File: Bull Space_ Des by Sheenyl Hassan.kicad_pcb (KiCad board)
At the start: 2 copper layers, 20 parts, among them IC1 TEENSY_4.0, IC2 XB24CZ7PIT-004, J1 Screw_Terminal_01x02, J2 Screw_Terminal_01x02, U1 Regulator_Linear_AP2204RB-3.3, U2 Flight-Computer_Adafruit_GPS_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, U3 ADXL343, U4 BMP280, U6 Memory_Flash_W25Q32JVSS

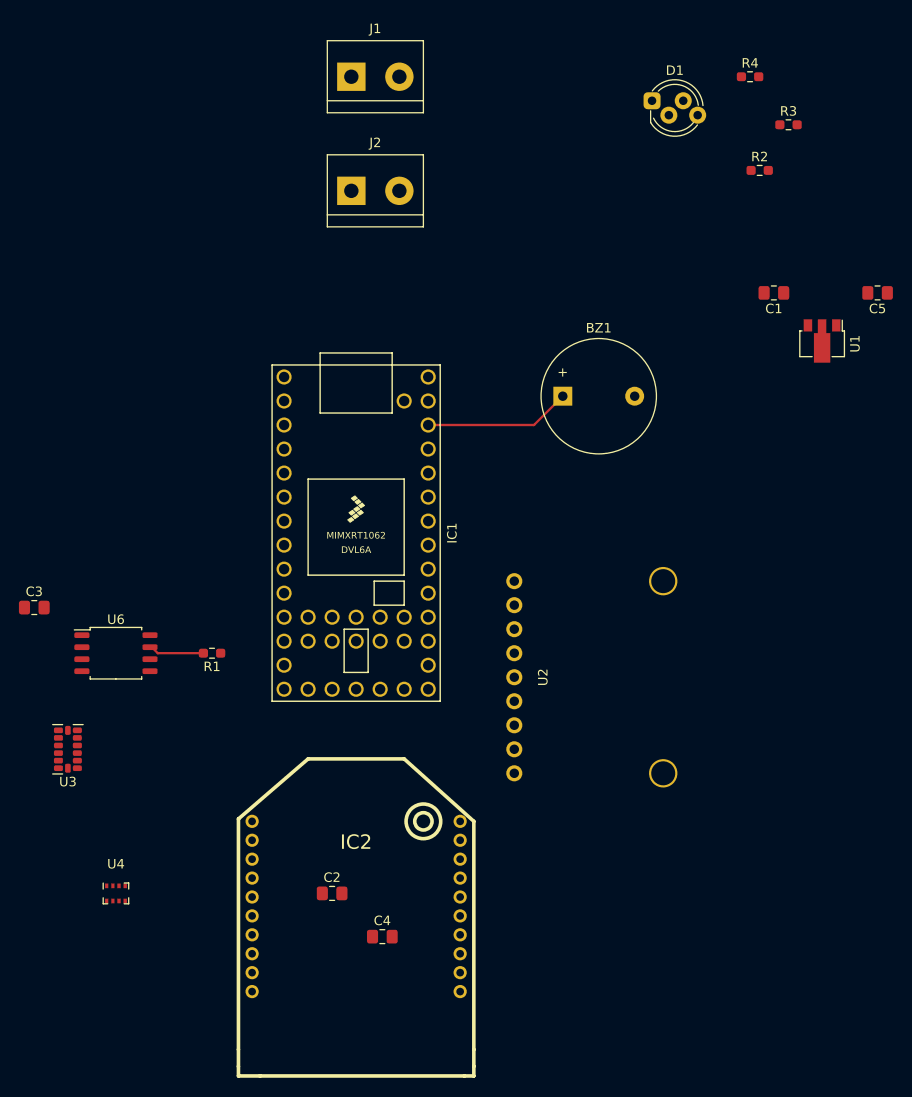
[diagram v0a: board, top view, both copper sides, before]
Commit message: Board Layout (kinda)
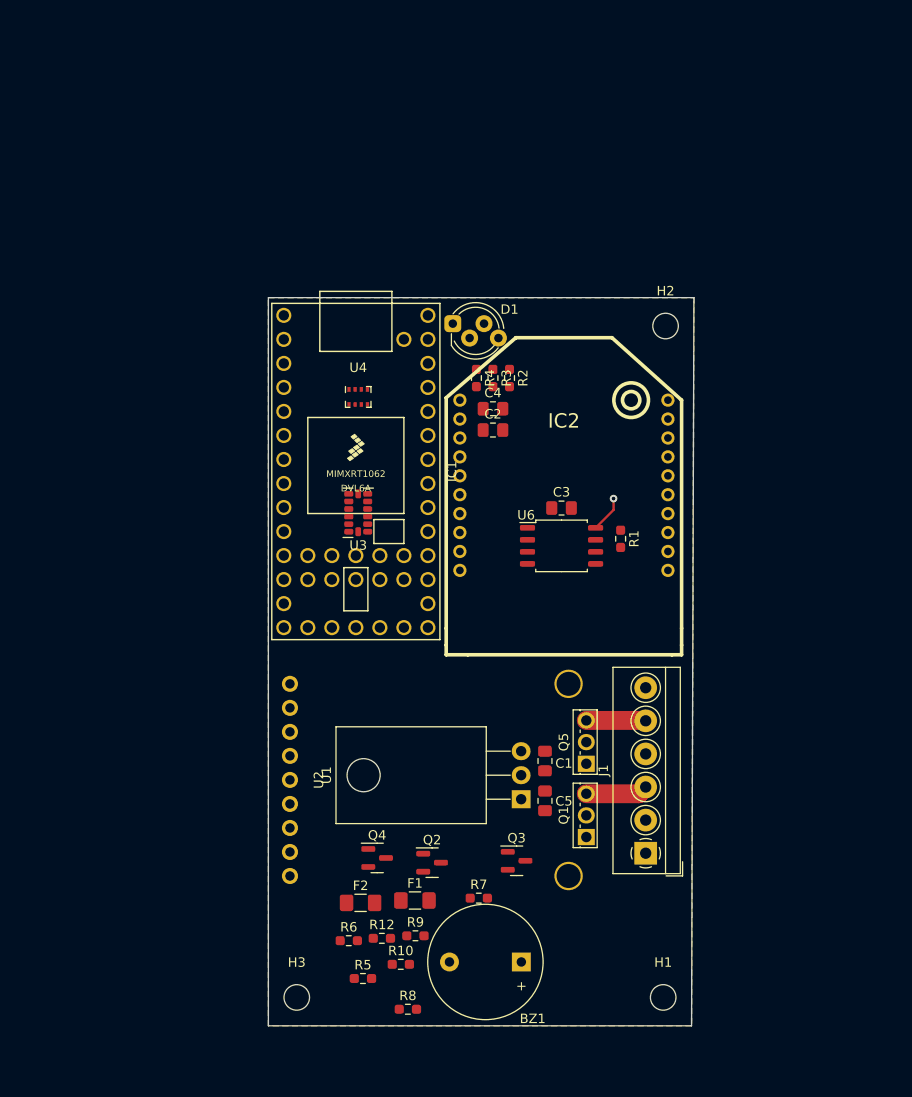
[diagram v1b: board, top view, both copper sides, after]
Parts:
- removed J2: Screw_Terminal_01x02, TerminalBlock:TerminalBlock_bornier-2_P5.08mm
- added F1: 3A Polyfuse, Fuse:Fuse_1206_3216Metric_Pad1.42x1.75mm_HandSolder, F.Cu at (87.5, 127.8)
- added F2: 3A Polyfuse, Fuse:Fuse_1206_3216Metric_Pad1.42x1.75mm_HandSolder, F.Cu at (81.8, 128.0)
- added H1: MountingHole, MountingHole:MountingHole_2.7mm_M2.5, F.Cu at (113.8, 138.0)
- added H2: MountingHole, MountingHole:MountingHole_2.7mm_M2.5, F.Cu at (114.0, 67.0)
- added H3: MountingHole, MountingHole:MountingHole_2.7mm_M2.5, F.Cu at (75.0, 138.0)
- added Q1: AOI21357, Package_TO_SOT_THT:TO-251-3_Vertical, F.Cu at (105.6, 121.0)
- added Q2: 2N7002, Package_TO_SOT_SMD:SOT-23, F.Cu at (89.3, 123.8)
- added Q3: 2N7002, Package_TO_SOT_SMD:SOT-23, F.Cu at (98.2, 123.5)
- added Q4: 2N7002, Package_TO_SOT_SMD:SOT-23, F.Cu at (83.5, 123.2)
- added Q5: AOI21357, Package_TO_SOT_THT:TO-251-3_Vertical, F.Cu at (105.6, 113.3)
- added R10: 10k, Resistor_SMD:R_0603_1608Metric_Pad0.98x0.95mm_HandSolder, F.Cu at (86.0, 134.5)
- added R12: 10k, Resistor_SMD:R_0603_1608Metric_Pad0.98x0.95mm_HandSolder, F.Cu at (84.0, 131.8)
- added R5: 100R, Resistor_SMD:R_0603_1608Metric_Pad0.98x0.95mm_HandSolder, F.Cu at (82.0, 136.0)
- added R6: 100R, Resistor_SMD:R_0603_1608Metric_Pad0.98x0.95mm_HandSolder, F.Cu at (80.5, 132.0)
- added R7: 100, Resistor_SMD:R_0603_1608Metric_Pad0.98x0.95mm_HandSolder, F.Cu at (94.2, 127.5)
- added R8: 10k, Resistor_SMD:R_0603_1608Metric_Pad0.98x0.95mm_HandSolder, F.Cu at (86.8, 139.2)
- added R9: 10k, Resistor_SMD:R_0603_1608Metric_Pad0.98x0.95mm_HandSolder, F.Cu at (87.5, 131.5)
- C1: value 1uf -> 10uf
- J1: value Screw_Terminal_01x02 -> Screw_Terminal_01x06; footprint TerminalBlock:TerminalBlock_bornier-2_P5.08mm -> TerminalBlock_4Ucon:TerminalBlock_4Ucon_1x06_P3.50mm_Horizontal
- U1: value Regulator_Linear_AP2204RB-3.3 -> VXO7803-1000; footprint Package_TO_SOT_SMD:SOT-89-3 -> Package_TO_SOT_THT:TO-220-3_Horizontal_TabDown
- U2: footprint Flight Computer:Adafruit_ADXL345_THT -> Flight Computer:Adafruit_GPS_THT
- moved J1 87.8 mm to (111.9, 122.8), turned to 90 degrees
- moved C5 64.2 mm to (101.2, 117.2), turned to 90 degrees
- moved BZ1 60.0 mm to (98.8, 134.2), turned to 180 degrees
- moved U4 58.4 mm to (81.5, 74.5)
- moved U1 58.0 mm to (98.7, 117.0), turned to 90 degrees
- moved C4 57.0 mm to (95.8, 75.8)
- moved C3 56.7 mm to (103.0, 86.2)
- moved C1 55.1 mm to (101.2, 113.0), turned to -90 degrees
- moved C2 51.9 mm to (95.8, 78.0)
- moved IC2 49.7 mm to (103.2, 74.8)
- moved U6 48.5 mm to (103.0, 90.2)
- moved R1 44.9 mm to (109.2, 89.5), turned to -90 degrees
- moved R4 43.0 mm to (94.0, 72.5), turned to -90 degrees
- moved R3 41.2 mm to (95.8, 72.5), turned to -90 degrees
- moved U3 39.6 mm to (81.5, 86.8)
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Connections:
- BZ1 pad 2: GND -> Net-(BZ1-Pad2)
- C1 pad 1: +3V3 -> +BATT
- C5 pad 1: 12V -> +3V3
- IC1 pad 7: unconnected-(IC1-Pad7) -> BUZZER
- IC1 pad 8: unconnected-(IC1-Pad8) -> /ACT1
- IC1 pad 9: unconnected-(IC1-Pad9) -> /ACT2
- J1 pad 1: BATT+ -> +BATT
- U1 pad 1: 12V -> +3V3
- U1 pad 3: +3V3 -> +BATT
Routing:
- net +3V3: track 15.5 -> 3.88 mm, vias 0 -> 1
- net /DROGUE_POW: track 0.00 -> 6.57 mm
- net /MAIN_POW: track 0.00 -> 6.30 mm
- net Net-(R1-Pad2): track 5.91 -> 0.00 mm
- added copper zone on B.Cu, net +3V3
- added copper zone on F.Cu, net GND
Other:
- board outline added: 45 x 77 mm
